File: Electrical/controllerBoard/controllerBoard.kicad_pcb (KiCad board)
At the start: 2 copper layers, 84.7 x 56.4 mm, 41 parts, among them J1 CONN_01X03, J11 MicroFit_RA_06, J12 MicroFit_RA_06, J13 MicroFit_RA_06, J14 MicroFit_RA_06, J2 0.1in_Female_Socket_01x16, J3 CONN_02X03, J4 NanoFit_2, J5 CONN_01X03, J6 0.1in_Female_Socket_01x16, J7 CONN_01X03, J8 CONN_01X03, J9 CONN_01X03, U1 ATmega328P-AU_SPEEDEV, U2 LT1086-5.0, U3 LT1086-3.3, Y1 Crystal_SMD

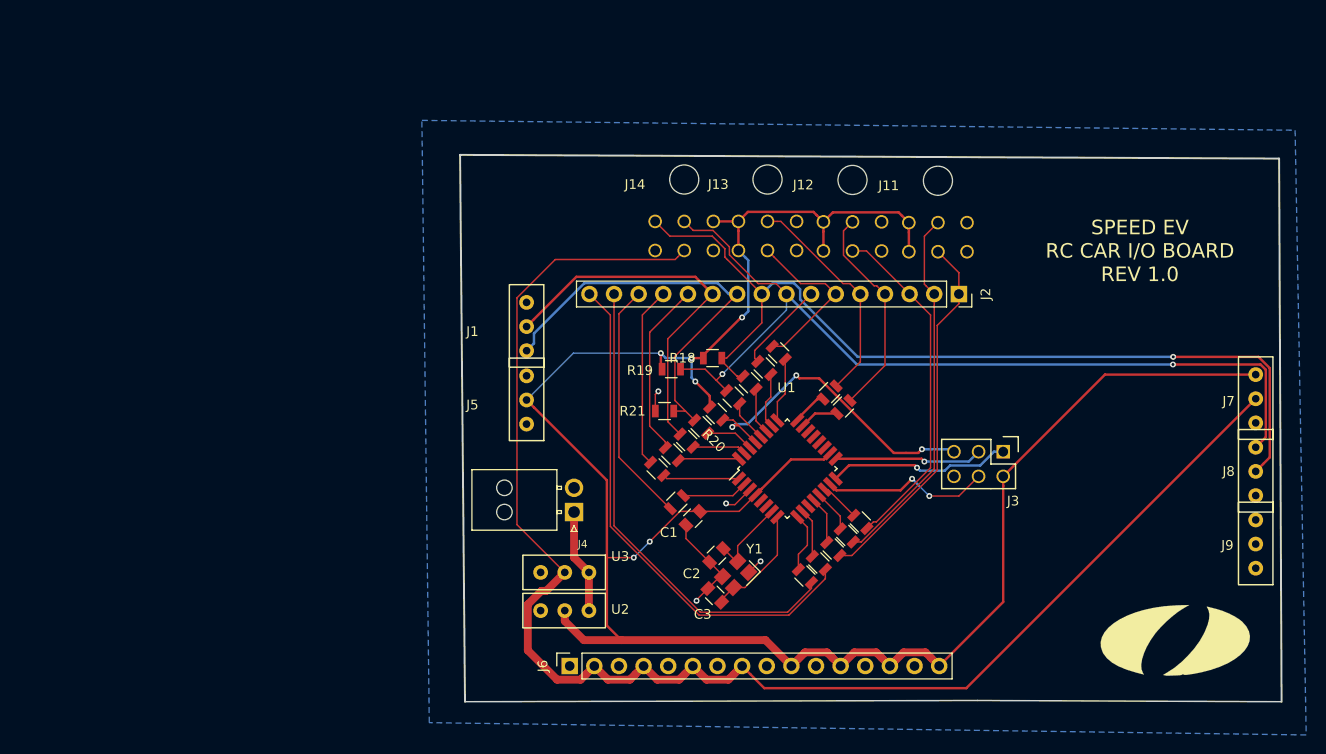
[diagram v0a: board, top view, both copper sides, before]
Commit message: updated controller board
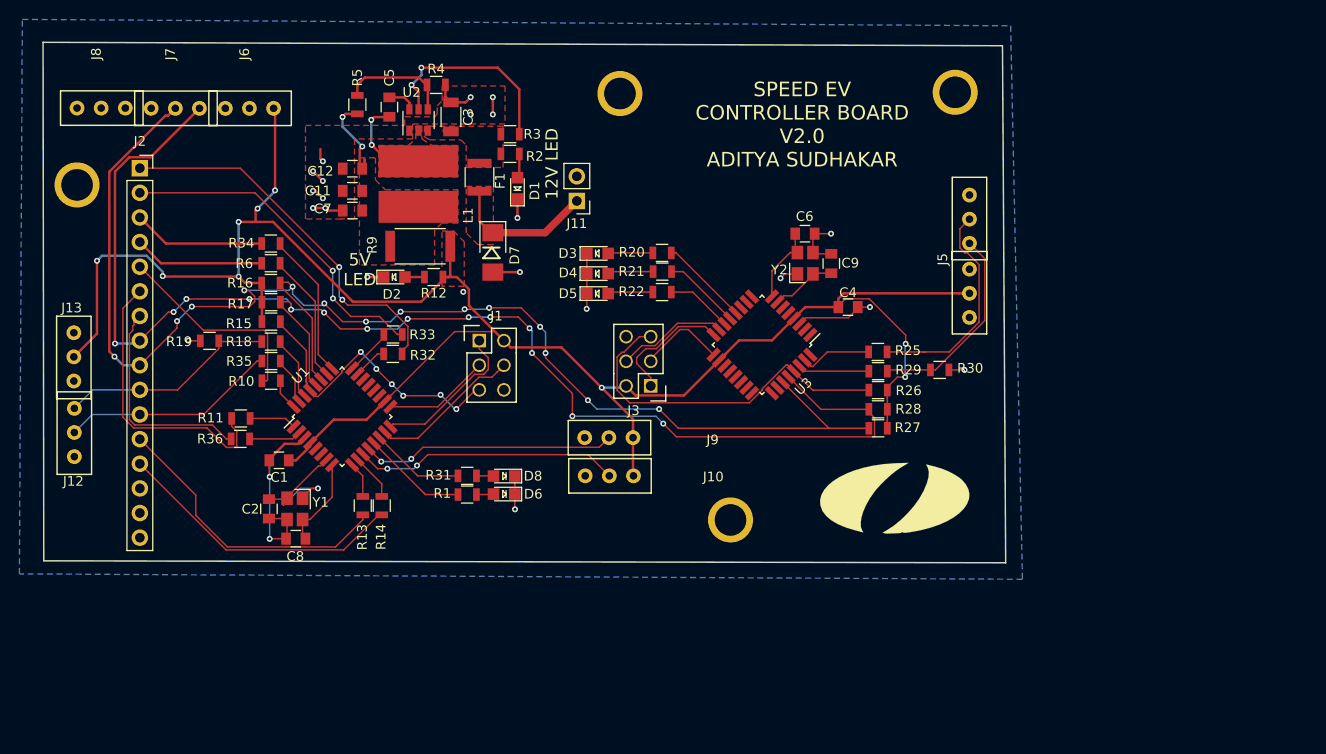
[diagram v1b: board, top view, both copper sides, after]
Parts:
- removed the G*** at (138.4, 110.7)
- removed J14: MicroFit_RA_06, footprints:MicroFit_RA_06
- removed R7, R8: R_0, footprints:R_0805_OEM
- added C11: C_1uF, footprints:C_0805_OEM, F.Cu at (53.7, 64.7)
- added C12: C_0.1uF, footprints:C_0805_OEM, F.Cu at (53.7, 62.4)
- added C4: C_0.1uF, footprints:C_0805_OEM, F.Cu at (104.8, 76.7)
- added C5: C_0.1uF, footprints:C_0805_OEM, F.Cu at (57.5, 56.0)
- added C6: C_30pF, footprints:C_0805_OEM, F.Cu at (100.3, 69.1)
- added C7: C_47uF, footprints:C_0805_OEM, F.Cu at (53.7, 66.7)
- added C8: C_30pF, footprints:C_0805_OEM, F.Cu at (47.8, 100.5)
- added C9: C_30pF, footprints:C_0805_OEM, F.Cu at (103.0, 72.2)
- added D1: LED_0805, footprints:LED_0805_OEM, F.Cu at (70.7, 64.4)
- added D2: LED_0805, footprints:LED_0805_OEM, F.Cu at (58.0, 73.6)
- added D3: LED_0805, footprints:LED_0805_OEM, F.Cu at (78.9, 71.1)
- added D4: LED_0805, footprints:LED_0805_OEM, F.Cu at (78.9, 73.2)
- added D5: LED_0805, footprints:LED_0805_OEM, F.Cu at (78.9, 75.3)
- added D6: LED_0805, footprints:LED_0805_OEM, F.Cu at (69.3, 95.9)
- added D7: D_Zener_18V, footprints:DO-214AA, F.Cu at (68.1, 71.0)
- added D8: LED_0805, footprints:LED_0805_OEM, F.Cu at (69.3, 94.1)
- added F1: 500mA, footprints:Fuse_1210, F.Cu at (66.8, 63.3)
- added G***: LOGO, footprints:Olin_O, F.Cu at (109.5, 96.1)
- added J10: CONN_01X03, footprints:MHSS1105, F.Cu at (80.2, 94.1)
- added L1: L_4.7uH, footprints:4.7uH_Inductor_OEM, F.Cu at (60.5, 64.0)
- added R11: R_0, footprints:R_0805_OEM, F.Cu at (42.2, 88.1)
- added R22: R_200, footprints:R_0805_OEM, F.Cu at (85.6, 75.1)
- added R25: R_0, footprints:R_0805_OEM, F.Cu at (107.8, 81.3)
- added R26: R_10K, footprints:R_0805_OEM, F.Cu at (107.9, 85.2)
- added R27: R_10K, footprints:R_0805_OEM, F.Cu at (107.9, 89.2)
- added R28: R_10K, footprints:R_0805_OEM, F.Cu at (107.9, 87.2)
- added R29: R_1K, footprints:R_0805_OEM, F.Cu at (107.9, 83.3)
- added R30: R_2.2K, footprints:R_0805_OEM, F.Cu at (114.2, 83.1)
- added R31: R_200, footprints:R_0805_OEM, F.Cu at (65.5, 94.1)
- added R32: R_0, footprints:R_0805_OEM, F.Cu at (57.8, 81.5)
- added R33: R_0, footprints:R_0805_OEM, F.Cu at (57.9, 79.5)
- added R34: R_0, footprints:R_0805_OEM, F.Cu at (45.3, 70.1)
- added R35: R_0, footprints:R_0805_OEM, F.Cu at (45.3, 82.2)
- added R36: R_0, footprints:R_0805_OEM, F.Cu at (42.1, 90.2)
- added REF**: Mounting_Hole_4-40, footprints:Mounting_Hole_4-40, F.Cu at (25.3, 64.1)
- added REF**: Mounting_Hole_4-40, footprints:Mounting_Hole_4-40, F.Cu at (92.7, 98.6)
- added REF**: Mounting_Hole_4-40, footprints:Mounting_Hole_4-40, F.Cu at (81.3, 54.6)
- added REF**: Mounting_Hole_4-40, footprints:Mounting_Hole_4-40, F.Cu at (115.8, 54.5)
- added Y2: Crystal_SMD, footprints:Crystal_SMD_FA238, F.Cu at (100.4, 72.1)
- C3: value C_30pF -> C_22uF; footprint footprints:C_0805_OEM -> footprints:C_1206_OEM
- J1: value CONN_01X03 -> CONN_02X03; footprint footprints:MHSS1105 -> footprints:Pin_Header_Straight_2x03
- J11: value MicroFit_RA_06 -> CONN_01x02; footprint footprints:MicroFit_RA_06 -> Connector_PinHeader_2.54mm:PinHeader_1x02_P2.54mm_Vertical
- J12, J13: value MicroFit_RA_06 -> CONN_01X03; footprint footprints:MicroFit_RA_06 -> footprints:MHSS1105
- J4: value NanoFit_2 -> CONN_01X03; footprint footprints:NanoFit_Molex_1x02x2.50mm_Angled_OEM -> footprints:MHSS1105
- J6: value 0.1in_Female_Socket_01x16 -> CONN_01X03; footprint Connector_PinSocket_2.54mm:PinSocket_1x16_P2.54mm_Vertical -> footprints:MHSS1105
- R1, R12: value R_0 -> R_200
- R10: value R_10K -> R_0
- R15, R16, R17: value R_0 -> R_10K
- R18: value R_10K -> R_1K
- R19: value R_10K -> R_2.2K
- R2: value R_0 -> R_1k
- R20: value R_1K -> R_200
- R21: value R_2.2K -> R_200
- R3, R4: value R_0 -> R_10k
- R5: value R_0 -> R_51.1k
- R9: value R_0 -> R_0_Jumper; footprint footprints:R_0805_OEM -> footprints:R_2512_OEM
- U1: value ATmega328P-AU_SPEEDEV -> ATmega328P-AU
- U2: value LT1086-5.0 -> TPS561201; footprint footprints:MHSS1105 -> footprints:SOT-23-6_OEM
- U3: value LT1086-3.3 -> ATmega328P-AU; footprint footprints:MHSS1105 -> Package_QFP:TQFP-32_7x7mm_P0.8mm
- moved J8 124.8 mm to (27.8, 56.1), turned to 270 degrees
- moved J7 115.4 mm to (35.4, 56.2), turned to 270 degrees
- moved J2 85.4 mm to (31.8, 62.3), turned to 0 degrees
- moved J12 84.4 mm to (25.0, 89.6), turned to 180 degrees
- moved J13 73.8 mm to (24.9, 81.8), turned to 180 degrees
- moved J9 67.6 mm to (80.1, 90.1), turned to 270 degrees
- moved J6 66.3 mm to (43.1, 56.2), turned to 270 degrees
- moved R16 62.8 mm to (45.3, 74.2), turned to 0 degrees
- moved R17 62.5 mm to (45.3, 76.1), turned to 0 degrees
- moved R5 57.0 mm to (54.2, 55.8), turned to 270 degrees
- moved C3 56.3 mm to (63.8, 57.0), turned to 90 degrees
- moved R3 53.9 mm to (69.9, 58.8), turned to 0 degrees
- moved R4 53.5 mm to (62.3, 53.7), turned to 0 degrees
- moved R6 53.2 mm to (45.3, 72.1), turned to 0 degrees
- moved U2 52.8 mm to (60.5, 57.4)
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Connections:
- net /IO12 renamed /IO8
- net /IO13 renamed /IO9
- C1 pad 1: +5V -> VCC
- C3 pad 1: /XTAL2 -> /12V_Fused
- J1 pad 1: Net-(J1-Pad1) -> /MISO
- J1 pad 2: /TX -> VCC
- J1 pad 3: /RX -> /SCK
- J11 pad 1: +5V -> +9V
- J11 pad 2: /IO2 -> GND
- J12 pad 1: +5V -> Net-(J12-Pad1)
- J12 pad 2: /IO4 -> /TX
- J12 pad 3: GND -> /RX
- J13 pad 1: +5V -> GND
- J13 pad 2: /IO5 -> VCC
- J13 pad 3: GND -> Net-(J13-Pad3)
- J2 pad 14: /IO14 -> Net-(J2-Pad14)
- J2 pad 15: /IO15 -> Net-(J2-Pad15)
- J2 pad 16: /IO16 -> Net-(J2-Pad16)
- J3 pad 1: /MISO -> /MISO2
- J3 pad 2: +5V -> VCC
- J3 pad 3: /SCK -> /SCK2
- J3 pad 4: /MOSI -> /MOSI2
- J3 pad 5: /RESET -> /RESET2
- J4 pad 1: /VIN_BAT -> Net-(J4-Pad1)
- J4 pad 2: GND -> /TX2
- J5 pad 2: +5V -> VCC
- J6 pad 1: GND -> VCC
- J6 pad 2: +3V3 -> Net-(J6-Pad2)
- J7 pad 1: +5V -> /SCL
- J7 pad 2: +3V3 -> /SDA
- J7 pad 3: GND -> Net-(J7-Pad3)
- J8 pad 1: /SCL -> Net-(J8-Pad1)
- J8 pad 2: /SDA -> Net-(J8-Pad2)
- J9 pad 1: Net-(J9-Pad1) -> VCC
- J9 pad 2: Net-(J9-Pad2) -> /THROTTLE_SENSE
- J9 pad 3: Net-(J9-Pad3) -> GND
- R1 pad 1: /IO1 -> Net-(D6-Pad2)
- R10 pad 1: +5V -> /IO5
- R10 pad 2: /RESET -> Net-(R10-Pad2)
- R12 pad 1: /TX -> VCC
- R12 pad 2: Net-(R12-Pad2) -> Net-(D2-Pad2)
- R15 pad 1: /IO14 -> VCC
- R15 pad 2: Net-(R15-Pad2) -> /RESET
- R16 pad 1: /IO15 -> VCC
- R16 pad 2: Net-(R16-Pad2) -> /SDA
- R17 pad 1: /IO16 -> VCC
- R17 pad 2: Net-(R17-Pad2) -> /SCL
- R18 pad 1: +5V -> /RX
- R18 pad 2: /SDA -> Net-(R18-Pad2)
- R19 pad 1: +5V -> GND
- R19 pad 2: /SCL -> /RX
- R2 pad 1: /IO2 -> /12V_Fused
- R2 pad 2: Net-(R2-Pad2) -> Net-(D1-Pad2)
- R20 pad 1: /RX -> Net-(D3-Pad2)
- R21 pad 1: GND -> Net-(D4-Pad2)
- R21 pad 2: /RX -> Net-(R21-Pad2)
- R3 pad 1: /IO3 -> /12V_Fused
- R4 pad 1: /IO4 -> Net-(R4-Pad1)
- R4 pad 2: Net-(R4-Pad2) -> GND
- R5 pad 1: /IO5 -> Net-(R4-Pad1)
- R5 pad 2: Net-(R5-Pad2) -> Net-(C11-Pad1)
- R6 pad 1: /IO6 -> /IO4
- R9 pad 1: /SCL -> VCC
- R9 pad 2: Net-(R9-Pad2) -> Net-(C11-Pad1)
- U1 pad 1: Net-(R14-Pad2) -> Net-(R11-Pad2)
- U1 pad 10: Net-(R17-Pad2) -> Net-(R14-Pad2)
- U1 pad 11: Net-(U1-Pad11) -> /STEERING_SENSE
- U1 pad 12: Net-(R1-Pad2) -> /THROTTLE_SENSE
- U1 pad 13: Net-(R2-Pad2) -> Net-(R1-Pad2)
- U1 pad 14: Net-(R3-Pad2) -> Net-(R31-Pad2)
- U1 pad 18: +5V -> VCC
- U1 pad 2: Net-(R15-Pad2) -> Net-(R36-Pad2)
- U1 pad 23: Net-(R4-Pad2) -> Net-(R32-Pad2)
- U1 pad 24: Net-(R5-Pad2) -> Net-(R33-Pad2)
- U1 pad 25: Net-(R6-Pad2) -> Net-(R34-Pad2)
- U1 pad 26: Net-(R7-Pad2) -> Net-(R6-Pad2)
- U1 pad 27: Net-(R8-Pad2) -> /SDA
- U1 pad 28: Net-(R9-Pad2) -> /SCL
- U1 pad 30: Net-(R20-Pad2) -> Net-(R18-Pad2)
- U1 pad 31: Net-(R12-Pad2) -> Net-(R35-Pad2)
- U1 pad 32: Net-(R13-Pad2) -> Net-(R10-Pad2)
- U1 pad 4: +5V -> VCC
- U1 pad 9: Net-(R16-Pad2) -> Net-(R13-Pad2)
- U2 pad 2: +5V -> Net-(C5-Pad2)
- U2 pad 3: /VIN_BAT -> /12V_Fused
- U3 pad 1: GND -> Net-(U3-Pad1)
- U3 pad 2: +3V3 -> Net-(U3-Pad2)
- U3 pad 3: /VIN_BAT -> GND
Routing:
- net +5V: track 226.4 -> 0.00 mm, vias 6 -> 0
- net VCC: track 0.00 -> 205.1 mm, vias 0 -> 9
- net +3V3: track 153.2 -> 0.00 mm
- net GND: track 17.7 -> 74.0 mm, vias 4 -> 25
- net /IO16: track 53.3 -> 0.00 mm
- net /SCL: track 92.8 -> 144.0 mm, vias 2 -> 14
- net /IO15: track 49.6 -> 0.00 mm
- net /SDA: track 94.7 -> 142.5 mm, vias 1 -> 14
- net /RESET2: track 0.00 -> 37.0 mm
- net /STEERING_SENSE: track 0.00 -> 27.5 mm, vias 0 -> 2
- net /THROTTLE_SENSE: track 0.00 -> 26.4 mm, vias 0 -> 2
- net /IO14: track 25.2 -> 0.00 mm
- net /TX2: track 0.00 -> 23.1 mm
- net /IO3: track 35.7 -> 13.7 mm
- net /RX2: track 0.00 -> 20.8 mm
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- added copper zone on F.Cu, net +9V
- added copper zone on F.Cu, net /12V_Fused
- added copper zone on F.Cu, net GND
- added copper zone on F.Cu, net Net-(C11-Pad1)
- added copper zone on F.Cu, net Net-(C5-Pad2)
- added copper zone on F.Cu, net VCC
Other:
- board size 84.7 x 56.4 mm -> 99.3 x 53.7 mm
- rule pad_to_mask_clearance: 0.051 -> 0.2
- board text added: "12V LED"
- board text added: "5V LED"
- board text added: "SPEED EV CONTROLLER BOARD V2.0 ADITYA SUDHAKAR"
- board text removed: "SPEED EV RC CAR I/O BOARD REV 1.0"
